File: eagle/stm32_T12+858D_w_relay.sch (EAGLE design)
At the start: 82 parts, among them IC1 REG1117, IC2 AD823, IC3 LM328, T1 BTA41 600B, U1 AT24C32A

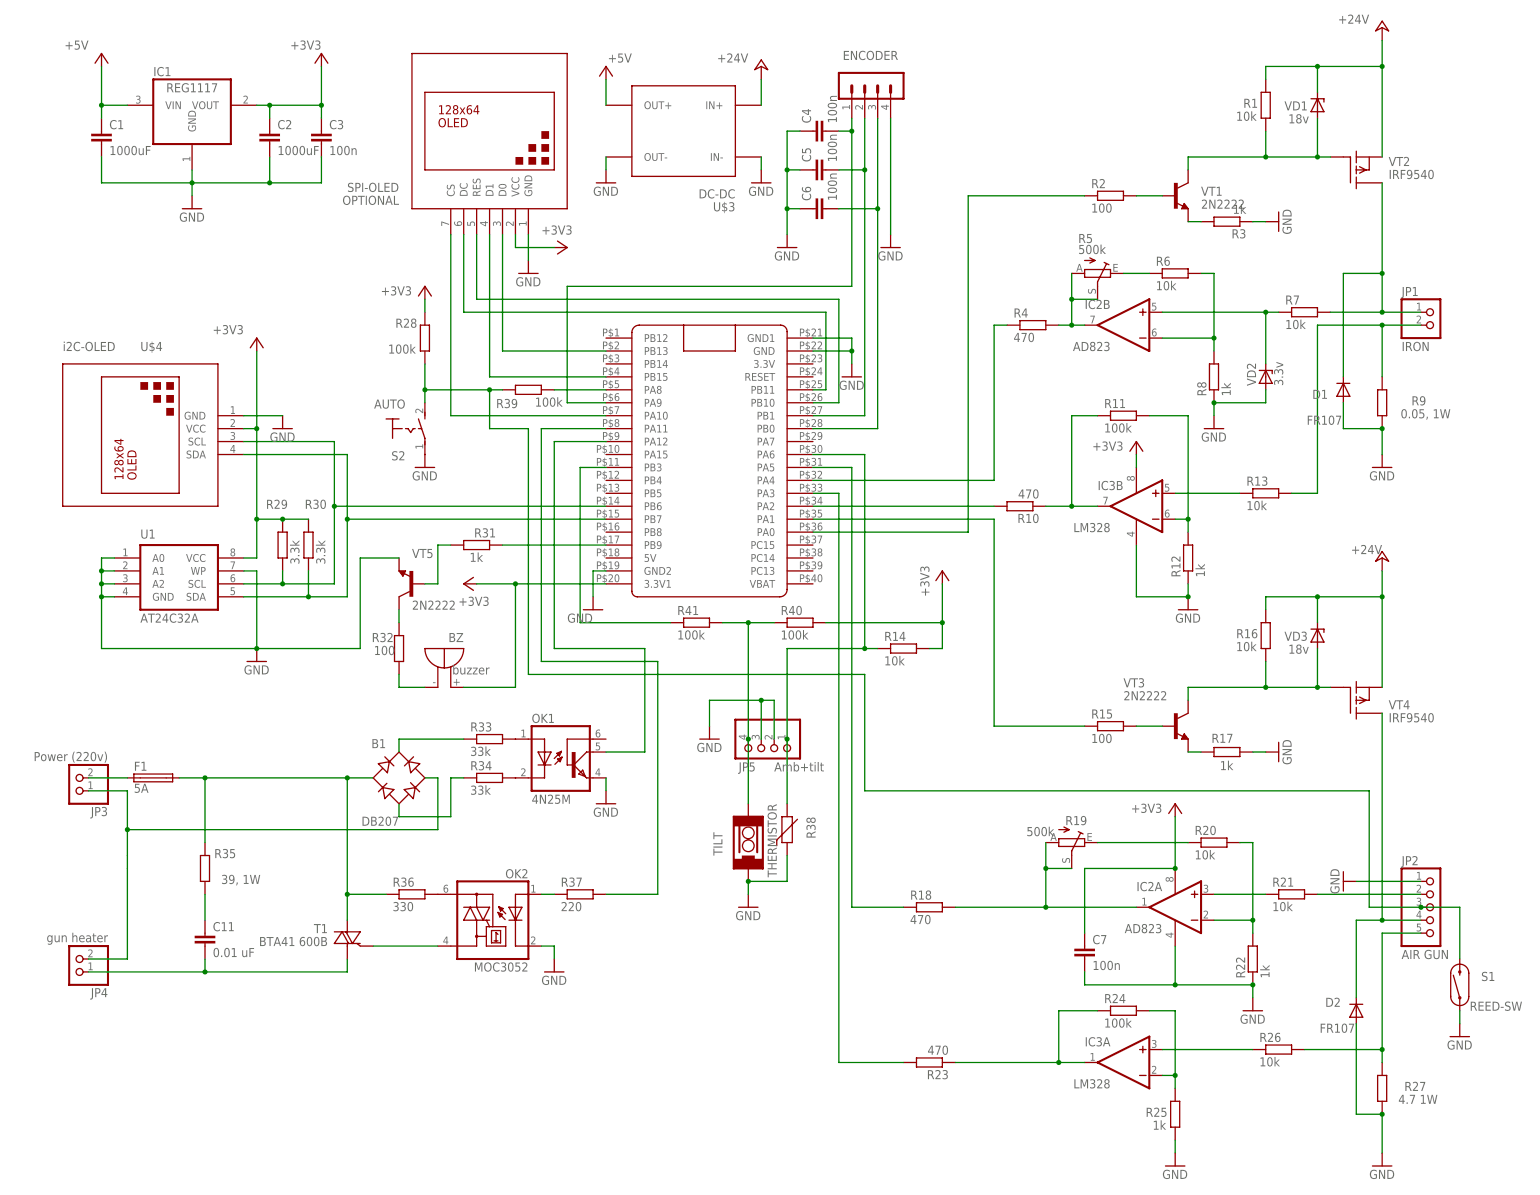
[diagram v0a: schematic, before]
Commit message: Add files via upload
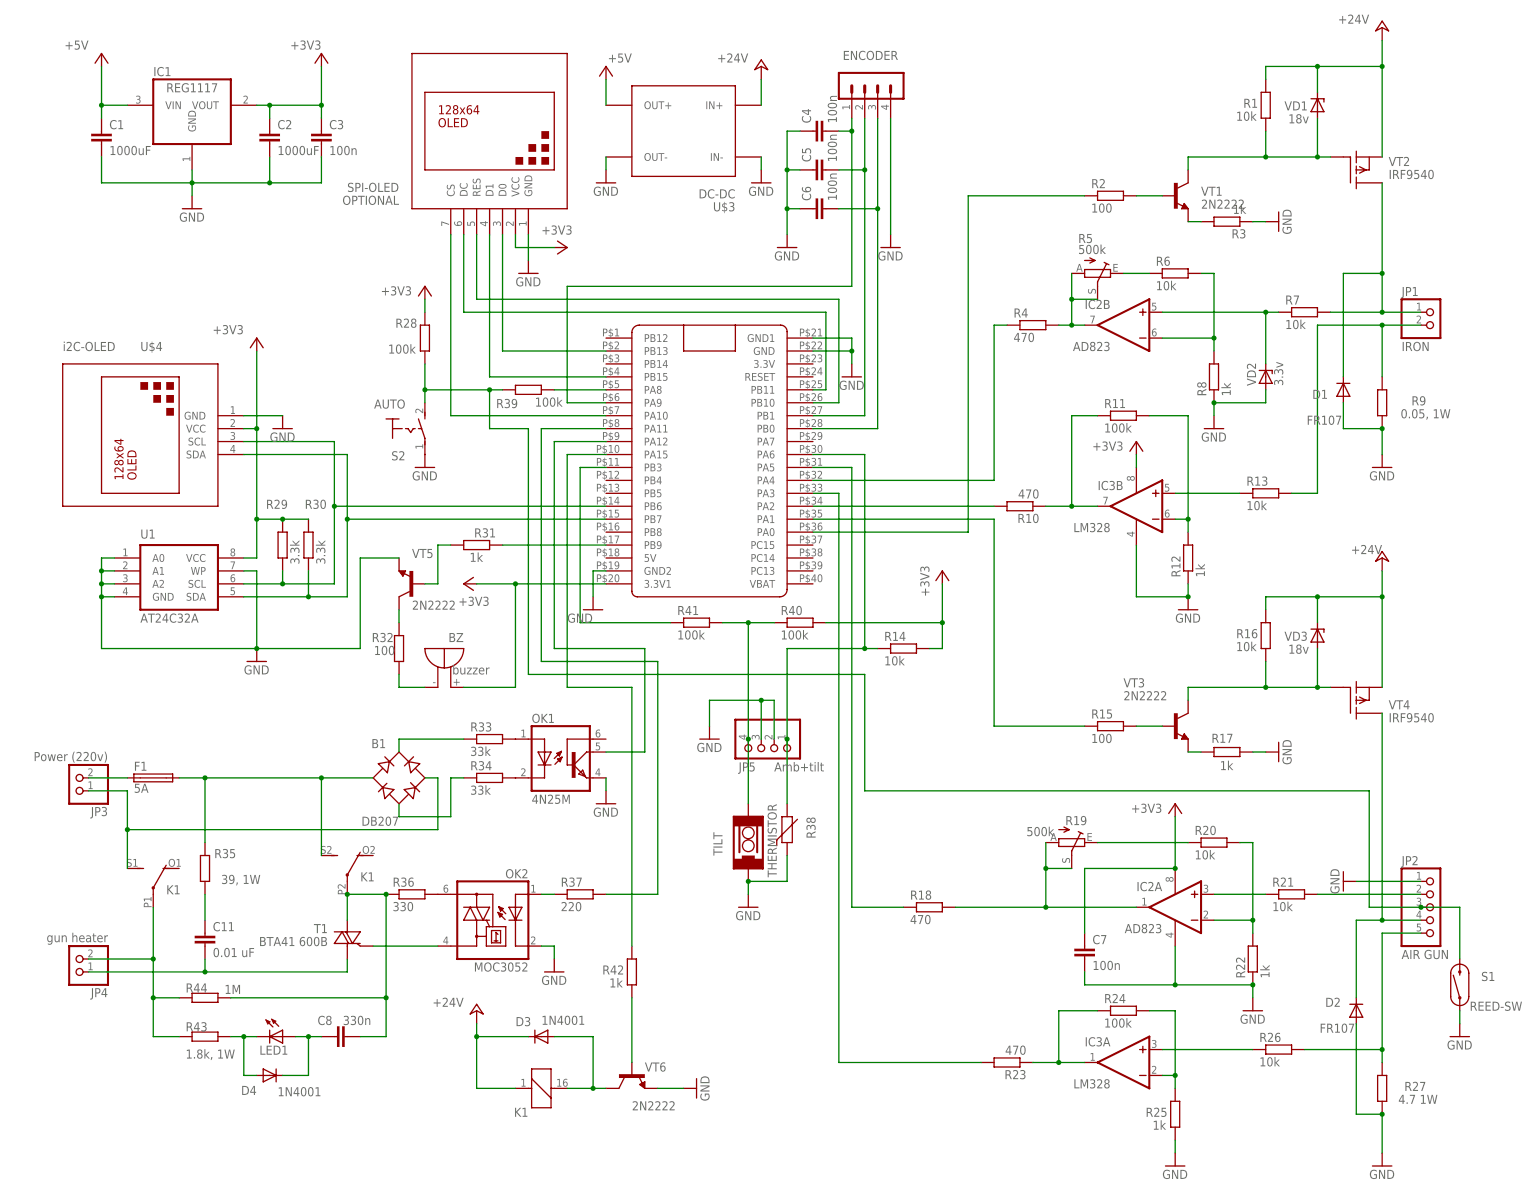
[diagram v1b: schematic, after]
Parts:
- added C8: 330n, rcl:C-EU025-025X050
- added D3, D4: 1N4001, diode:1N4004
- added K1: 351, relay:351
- added LED1: (no value), SparkFun:LED-3MM-NO_SILK
- added R42: 1k, rcl:R-EU_0204/5
- added R43: 1.8k, 1W, eagle-ltspice:R0204/7
- added R44: 1M, eagle-ltspice:R0204/7
- added VT6: 2N2222, transistor:2N2222
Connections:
- new net N$38: R42.1, VT6.B
- new net N$66: D3.A, K11.2, VT6.C
- new net N$67: R42.2, U$1.PA15
- new net N$68: JP4.2, K12.P, R43.2, R44.2
- new net N$69: C8.1, D4.C, LED1.A
- new net N$71: D4.A, LED1.C, R43.1
- new net N$72: C8.2, K13.P, R36.1, R44.1, T1.A2
- net +24V: now also D3.C, K11.1
- net GND: now also VT6.E
- net N$40: now also K12.S; no longer JP4.2
- net N$46: now also K13.S; no longer R36.1, T1.A2
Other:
- moved on the sheet: R23
